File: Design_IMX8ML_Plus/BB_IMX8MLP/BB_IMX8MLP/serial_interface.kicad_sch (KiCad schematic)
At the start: 1 part, among them U31 FT4232H

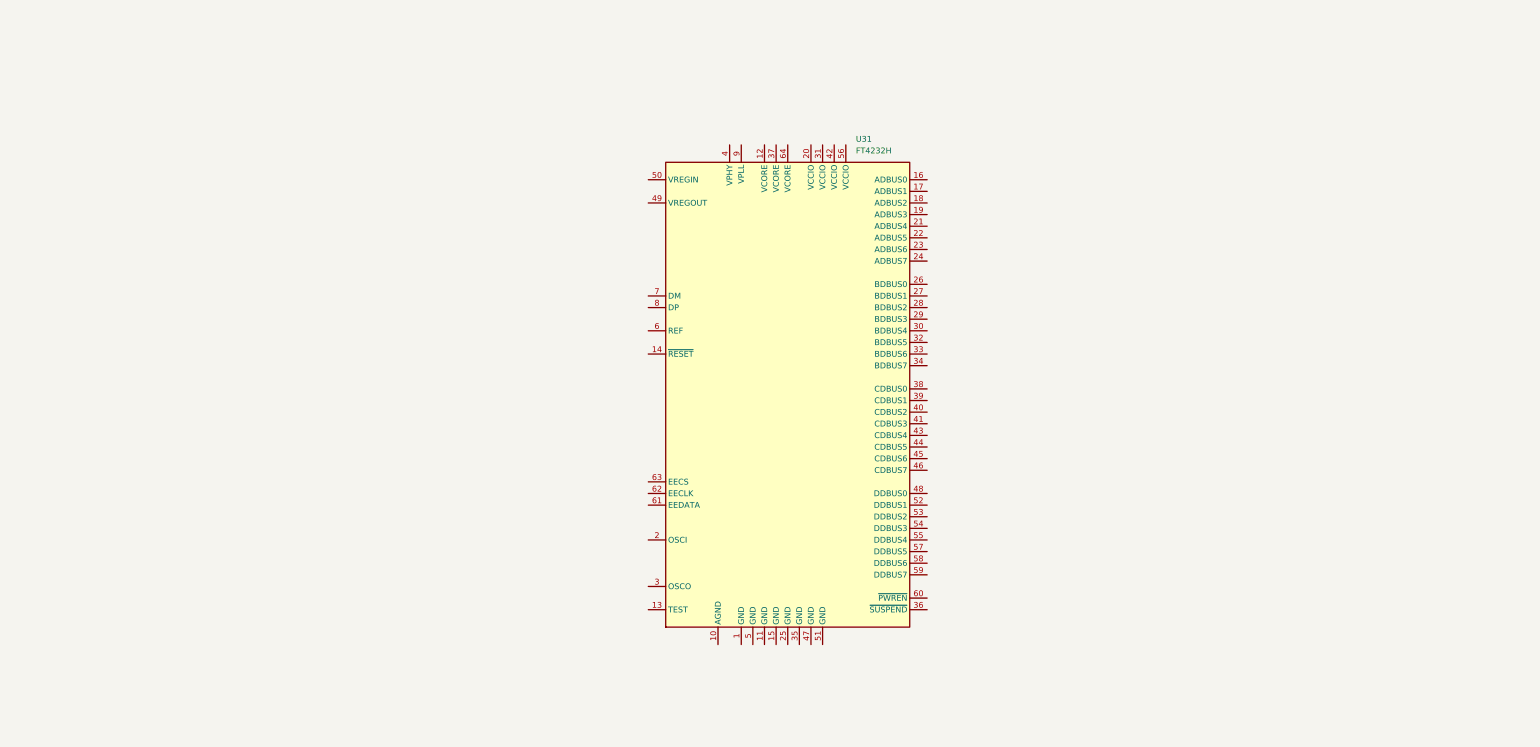
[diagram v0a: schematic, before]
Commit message: Review
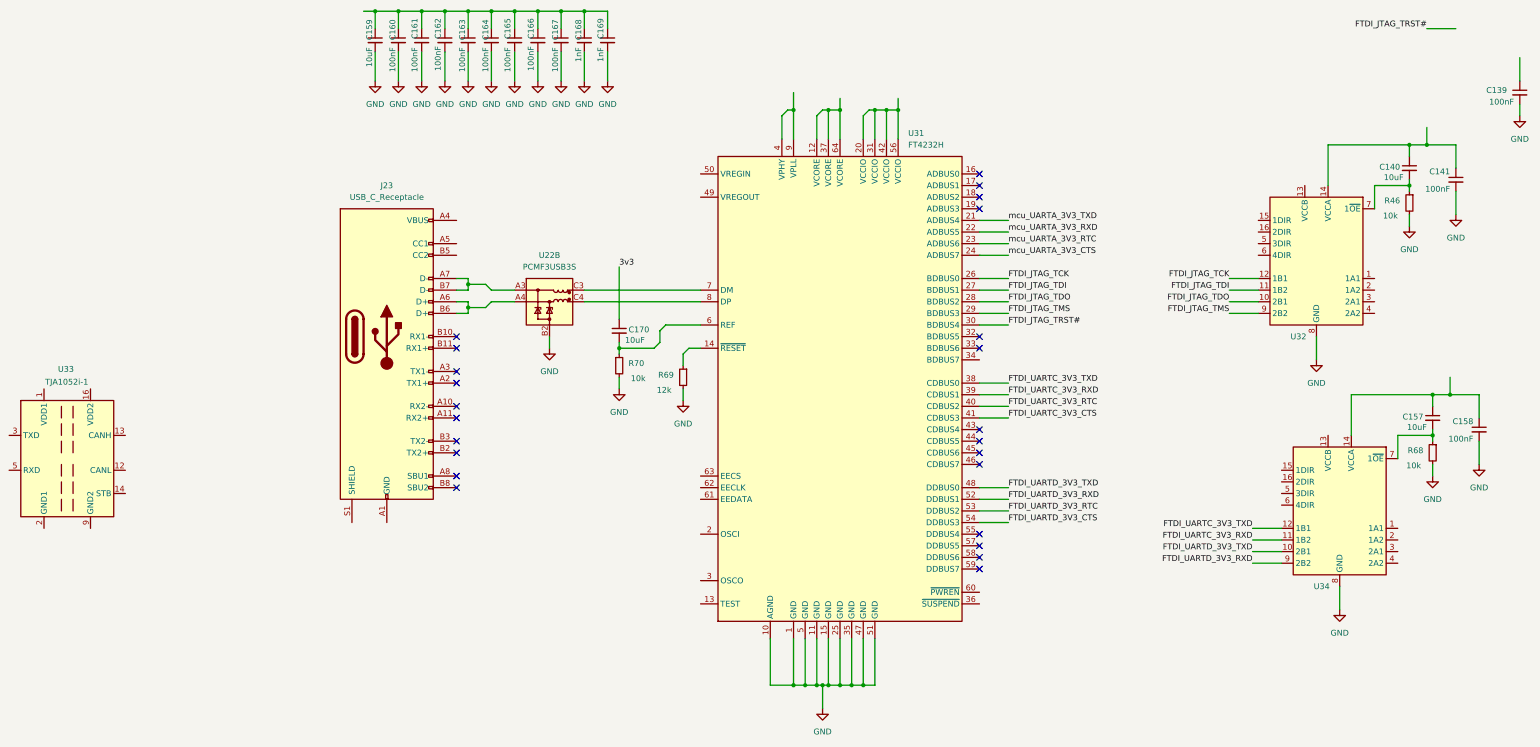
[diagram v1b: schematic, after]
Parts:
- added C139, C141, C158, C160, C161, C162, C163, C164, C165, C166, C167: 100nF, Capacitor_SMD:C_0402_1005Metric, symbol Device:C_Small
- added C140, C157, C159, C170: 10uF, Capacitor_SMD:C_0402_1005Metric, symbol Device:C_Small
- added C168, C169: 1nF, Capacitor_SMD:C_0402_1005Metric, symbol Device:C_Small
- added J23: USB_C_Receptacle, symbol Connector:USB_C_Receptacle
- added R46, R68, R70: 10k, Resistor_SMD:R_0402_1005Metric, symbol Device:R_Small
- added R69: 12k, Resistor_SMD:R_0402_1005Metric, symbol Device:R_Small
- added U22: PCMF3USB3S, Package_CSP:Nexperia_WLCSP-15_6-3-6_2.37x1.17mm_Layout6x3_P0.4mm, symbol Power_Protection:PCMF3USB3S
- added U32, U34: ~, symbol _W_MX8M:SN74AVC4T774RSVR
- added U33: TJA1052i-1, Package_SO:SOIC-16W_7.5x10.3mm_P1.27mm, symbol Interface_CAN_LIN:TJA1052i-1
- U31: footprint (none) -> Package_DFN_QFN:VQFN-64-1EP_9x9mm_P0.5mm_EP5.4x5.4mm
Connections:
- net GND: now reaches U31.1 (GND)
- net GND: now also U31.10 (AGND), U31.11 (GND), U31.15 (GND), U31.25 (GND), U31.35 (GND), U31.47 (GND), U31.5 (GND), U31.51 (GND), C139.2, C141.2, C158.2, C159.2, C160.2, C161.2, C162.2, C163.2, C164.2, C165.2, C166.2, C167.2, C168.2, C169.2, R46.2, R68.2, R69.2, R70.2, U22.B2 (GND_CH2), U32.8 (GND), U32.9 (GND), U34.8 (GND), U34.9 (GND)
- net at U31.12 (VCORE): now also U31.37 (VCORE), U31.64 (VCORE)
- net at U31.14 (~{RESET}): now also R69.1
- net at U31.20 (VCCIO): now also U31.31 (VCCIO), U31.42 (VCCIO), U31.56 (VCCIO)
- net mcu_UARTA_3V3_TXD: now reaches U31.21 (ADBUS4)
- net mcu_UARTA_3V3_RXD: now reaches U31.22 (ADBUS5)
- net mcu_UARTA_3V3_RTC: now reaches U31.23 (ADBUS6)
- net mcu_UARTA_3V3_CTS: now reaches U31.24 (ADBUS7)
- net FTDI_JTAG_TCK: now reaches U31.26 (BDBUS0)
- net FTDI_JTAG_TCK: now also U32.12 (1B1)
- net FTDI_JTAG_TDI: now reaches U31.27 (BDBUS1)
- net FTDI_JTAG_TDI: now also U32.11 (1B2)
- net FTDI_JTAG_TDO: now reaches U31.28 (BDBUS2)
- net FTDI_JTAG_TDO: now also U32.10 (2B1)
- net FTDI_JTAG_TMS: now reaches U31.29 (BDBUS3)
- net FTDI_JTAG_TMS: now also U32.9 (GND)
- net FTDI_JTAG_TRST#: now reaches U31.30 (BDBUS4)
- net FTDI_UARTC_3V3_TXD: now reaches U31.38 (CDBUS0)
- net FTDI_UARTC_3V3_TXD: now also U34.12 (1B1)
- net FTDI_UARTC_3V3_RXD: now reaches U31.39 (CDBUS1)
- net FTDI_UARTC_3V3_RXD: now also U34.11 (1B2)
- net at U31.4 (VPHY): now also U31.9 (VPLL)
- net FTDI_UARTC_3V3_RTC: now reaches U31.40 (CDBUS2)
- net FTDI_UARTC_3V3_CTS: now reaches U31.41 (CDBUS3)
- net FTDI_UARTD_3V3_TXD: now reaches U31.48 (DDBUS0)
- net FTDI_UARTD_3V3_TXD: now also U34.10 (2B1)
- net FTDI_UARTD_3V3_RXD: now reaches U31.52 (DDBUS1)
- net FTDI_UARTD_3V3_RXD: now also U34.9 (GND)
- net FTDI_UARTD_3V3_RTC: now reaches U31.53 (DDBUS2)
- net FTDI_UARTD_3V3_CTS: now reaches U31.54 (DDBUS3)
- net at U31.6 (REF): now also C170.2, R70.1
- net at U31.7 (DM): now also U22.C3 (CH2_OUT+)
- net at U31.8 (DP): now also U22.C4 (CH2_OUT-)
- new net: C157.1, C158.1, U34.14 (VCCA)
- new net: C157.2, R68.1, U34.7 (1~{OE})
- new net: J23.A7 (D-), J23.B7 (D-), U22.A3 (CH2_IN+)
- new net: J23.A6 (D+), J23.B6 (D+), U22.A4 (CH2_IN-)
- new net: U33.10 (GND2), U33.15 (GND2), U33.9 (GND2)
- new net: U33.11 (VDD2), U33.16 (VDD2)
- new net: U33.2 (GND1), U33.7 (GND1), U33.8 (GND1)
- new net: C159.1, C160.1, C161.1, C162.1, C163.1, C164.1, C165.1, C166.1, C167.1, C168.1, C169.1
- new net: C140.1, C141.1, U32.14 (VCCA)
- new net: C140.2, R46.1, U32.7 (1~{OE})
- new net: J23.A1 (GND), J23.A12 (GND), J23.B1 (GND), J23.B12 (GND)
- new net: J23.A4 (VBUS), J23.A9 (VBUS), J23.B4 (VBUS), J23.B9 (VBUS)
- new net 3v3: C170.1
- no-connect marks 0 -> 24
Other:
- moved on the sheet: U31
